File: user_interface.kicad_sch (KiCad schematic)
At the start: 11 parts, among them J4 B4B-XH-AM, J6 Conn_01x05, Q2 BC817, Q3 BC817

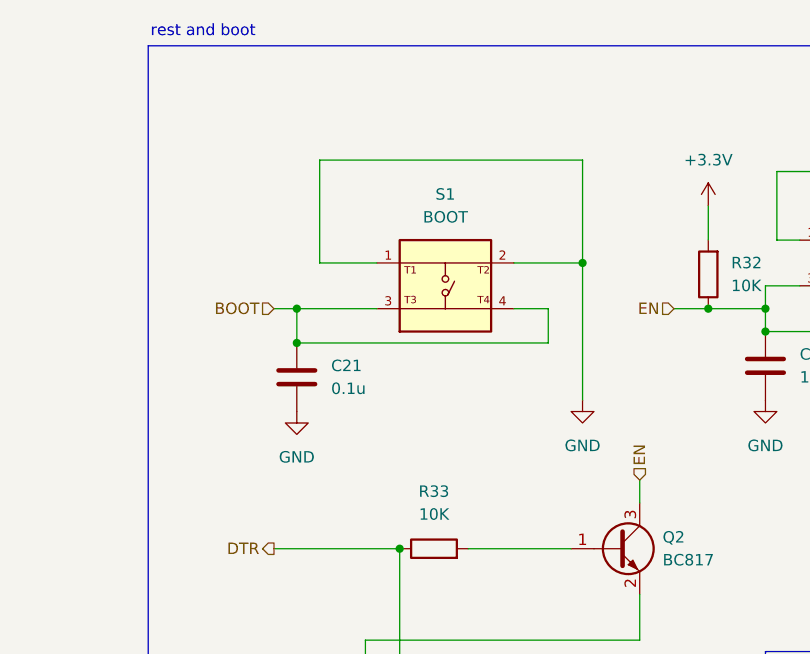
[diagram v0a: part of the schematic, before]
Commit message: intial_PCB
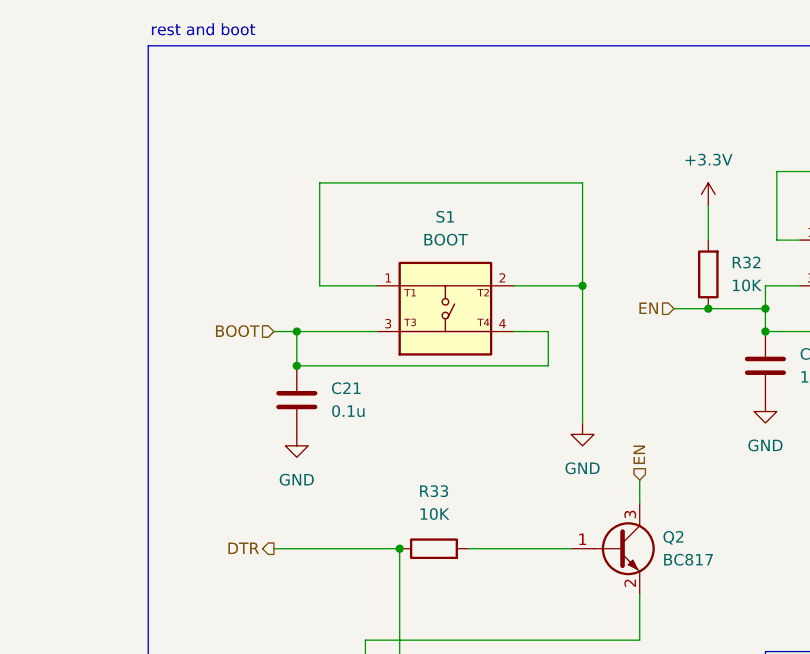
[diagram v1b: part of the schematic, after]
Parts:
- S1, S2: footprint USLPT2819DT2TR:SW_USLPT2819DT2TR -> Footprints:SW_USLPT2819DT2TR
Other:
- moved on the sheet: C21, S1
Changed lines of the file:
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@@
 	)
 	(junction
-		(at 163.83 58.42)
+		(at 163.83 60.96)
 		(diameter 0)
 		(color 0 0 0 0)
@@
 	)
 	(junction
-		(at 132.08 63.5)
+		(at 132.08 66.04)
 		(diameter 0)
 		(color 0 0 0 0)
@@
 	)
 	(junction
-		(at 132.08 67.31)
+		(at 132.08 69.85)
 		(diameter 0)
 		(color 0 0 0 0)
@@
 	(wire
 		(pts
-			(xy 163.83 58.42) (xy 163.83 73.66)
+			(xy 163.83 60.96) (xy 163.83 76.2)
 		)
 		(stroke
@@
 	(wire
 		(pts
-			(xy 129.54 63.5) (xy 132.08 63.5)
+			(xy 129.54 66.04) (xy 132.08 66.04)
 		)
 		(stroke
@@
 	(wire
 		(pts
-			(xy 134.62 46.99) (xy 163.83 46.99)
+			(xy 134.62 49.53) (xy 163.83 49.53)
 		)
 		(stroke
@@
 	(wire
 		(pts
-			(xy 140.97 58.42) (xy 134.62 58.42)
+			(xy 140.97 60.96) (xy 134.62 60.96)
 		)
 		(stroke
@@
 	(wire
 		(pts
-			(xy 132.08 63.5) (xy 140.97 63.5)
+			(xy 132.08 66.04) (xy 140.97 66.04)
 		)
 		(stroke
@@
 	(wire
 		(pts
-			(xy 163.83 46.99) (xy 163.83 58.42)
-		)
-		(stroke
-			(width 0)
-			(type default)
-		)
-	)
-	(wire
-		(pts
-			(xy 160.02 67.31) (xy 132.08 67.31)
-		)
-		(stroke
-			(width 0)
-			(type default)
-		)
-	)
-	(wire
-		(pts
-			(xy 132.08 63.5) (xy 132.08 67.31)
-		)
-		(stroke
-			(width 0)
-			(type default)
-		)
-	)
-	(wire
-		(pts
-			(xy 156.21 58.42) (xy 163.83 58.42)
+			(xy 163.83 49.53) (xy 163.83 60.96)
+		)
+		(stroke
+			(width 0)
+			(type default)
+		)
+	)
+	(wire
+		(pts
+			(xy 160.02 69.85) (xy 132.08 69.85)
+		)
+		(stroke
+			(width 0)
+			(type default)
+		)
+	)
+	(wire
+		(pts
+			(xy 132.08 66.04) (xy 132.08 69.85)
+		)
+		(stroke
+			(width 0)
+			(type default)
+		)
+	)
+	(wire
+		(pts
+			(xy 156.21 60.96) (xy 163.83 60.96)
 		)
 		(stroke
@@
 	(wire
 		(pts
-			(xy 134.62 58.42) (xy 134.62 46.99)
-		)
-		(stroke
-			(width 0)
-			(type default)
-		)
-	)
-	(wire
-		(pts
-			(xy 156.21 63.5) (xy 160.02 63.5)
-		)
-		(stroke
-			(width 0)
-			(type default)
-		)
-	)
-	(wire
-		(pts
-			(xy 160.02 63.5) (xy 160.02 67.31)
+			(xy 134.62 60.96) (xy 134.62 49.53)
+		)
+		(stroke
+			(width 0)
+			(type default)
+		)
+	)
+	(wire
+		(pts
+			(xy 156.21 66.04) (xy 160.02 66.04)
+		)
+		(stroke
+			(width 0)
+			(type default)
+		)
+	)
+	(wire
+		(pts
+			(xy 160.02 66.04) (xy 160.02 69.85)
 		)
 		(stroke
@@
 	(hierarchical_label "BOOT"
 		(shape input)
-		(at 129.54 63.5 180)
+		(at 129.54 66.04 180)
 		(effects
 			(font
@@
 	(symbol
 		(lib_id "USLPT2819DT2TR:USLPT2819DT2TR")
-		(at 148.59 60.96 0)
+		(at 148.59 63.5 0)
 		(unit 1)
 		(exclude_from_sim no)
@@
 		(fields_autoplaced yes)
 		(property "Reference" "S1"
-			(at 148.59 50.8 0)
+			(at 148.59 53.34 0)
 			(effects
 				(font
@@
 		)
 		(property "Value" "BOOT"
-			(at 148.59 53.34 0)
-			(effects
-				(font
-					(size 1.27 1.27)
-				)
-			)
-		)
-		(property "Footprint" "USLPT2819DT2TR:SW_USLPT2819DT2TR"
-			(at 148.59 60.96 0)
+			(at 148.59 55.88 0)
+			(effects
+				(font
+					(size 1.27 1.27)
+				)
+			)
+		)
+		(property "Footprint" "Footprints:SW_USLPT2819DT2TR"
+			(at 148.59 63.5 0)
 			(effects
 				(font
@@
 		)
 		(property "Datasheet" ""
-			(at 148.59 60.96 0)
+			(at 148.59 63.5 0)
 			(effects
 				(font
@@
 		)
 		(property "Description" ""
-			(at 148.59 60.96 0)
+			(at 148.59 63.5 0)
 			(effects
 				(font
@@
 		)
 		(property "MF" "TE Connectivity"
-			(at 148.59 60.96 0)
+			(at 148.59 63.5 0)
 			(effects
 				(font
@@
 		)
 		(property "Description_1" "Tactile Switch SPST-NO Top Actuated Surface Mount"
-			(at 148.59 60.96 0)
+			(at 148.59 63.5 0)
 			(effects
 				(font
@@
 		)
 		(property "Package" "None"
-			(at 148.59 60.96 0)
+			(at 148.59 63.5 0)
 			(effects
 				(font
@@
 		)
 		(property "Price" "None"
-			(at 148.59 60.96 0)
+			(at 148.59 63.5 0)
 			(effects
 				(font
@@
 		)
 		(property "Check_prices" "https://www.snapeda.com/parts/USLPT2819DT2TR/TE+Connectivity+ALCOSWITCH+Switches/view-part/?ref=eda"
-			(at 148.59 60.96 0)
+			(at 148.59 63.5 0)
 			(effects
 				(font
@@
 		)
 		(property "STANDARD" "Manufacturer Recommendations"
-			(at 148.59 60.96 0)
+			(at 148.59 63.5 0)
 			(effects
 				(font
@@
 		)
 		(property "PARTREV" "P"
-			(at 148.59 60.96 0)
+			(at 148.59 63.5 0)
 			(effects
 				(font
@@
 		)
 		(property "SnapEDA_Link" "https://www.snapeda.com/parts/USLPT2819DT2TR/TE+Connectivity+ALCOSWITCH+Switches/view-part/?ref=snap"
-			(at 148.59 60.96 0)
+			(at 148.59 63.5 0)
 			(effects
 				(font
@@
 		)
 		(property "MP" "USLPT2819DT2TR"
-			(at 148.59 60.96 0)
+			(at 148.59 63.5 0)
 			(effects
 				(font
@@
 		)
 		(property "Availability" "In Stock"
-			(at 148.59 60.96 0)
+			(at 148.59 63.5 0)
 			(effects
 				(font
@@
 		)
 		(property "MANUFACTURER" "TE CONNECTIVITY"
-			(at 148.59 60.96 0)
+			(at 148.59 63.5 0)
 			(effects
 				(font
@@
 	(symbol
 		(lib_id "power:GND")
-		(at 132.08 74.93 0)
+		(at 132.08 77.47 0)
 		(unit 1)
 		(exclude_from_sim no)
@@
 		(fields_autoplaced yes)
 		(property "Reference" "#PWR055"
-			(at 132.08 81.28 0)
+			(at 132.08 83.82 0)
 			(effects
 				(font
@@
 		)
 		(property "Value" "GND"
-			(at 132.08 80.01 0)
+			(at 132.08 82.55 0)
 			(effects
 				(font
@@
 		)
 		(property "Footprint" ""
-			(at 132.08 74.93 0)
+			(at 132.08 77.47 0)
 			(effects
 				(font
@@
 		)
 		(property "Datasheet" ""
-			(at 132.08 74.93 0)
+			(at 132.08 77.47 0)
 			(effects
 				(font
@@
 		)
 		(property "Description" "Power symbol creates a global label with name \"GND\" , ground"
-			(at 132.08 74.93 0)
+			(at 132.08 77.47 0)
 			(effects
 				(font
@@
 			)
 		)
-		(property "Footprint" "USLPT2819DT2TR:SW_USLPT2819DT2TR"
+		(property "Footprint" "Footprints:SW_USLPT2819DT2TR"
 			(at 195.58 58.42 0)
 			(effects
@@
 	(symbol
 		(lib_id "power:GND")
-		(at 163.83 73.66 0)
+		(at 163.83 76.2 0)
 		(unit 1)
 		(exclude_from_sim no)
@@
 		(fields_autoplaced yes)
 		(property "Reference" "#PWR050"
-			(at 163.83 80.01 0)
+			(at 163.83 82.55 0)
 			(effects
 				(font
@@
 		)
 		(property "Value" "GND"
-			(at 163.83 78.74 0)
+			(at 163.83 81.28 0)
 			(effects
 				(font
@@
 		)
 		(property "Footprint" ""
-			(at 163.83 73.66 0)
+			(at 163.83 76.2 0)
 			(effects
 				(font
@@
 		)
 		(property "Datasheet" ""
-			(at 163.83 73.66 0)
+			(at 163.83 76.2 0)
 			(effects
 				(font
@@
 		)
 		(property "Description" "Power symbol creates a global label with name \"GND\" , ground"
-			(at 163.83 73.66 0)
+			(at 163.83 76.2 0)
 			(effects
 				(font
@@
 	(symbol
 		(lib_id "Device:C")
-		(at 132.08 71.12 0)
+		(at 132.08 73.66 0)
 		(unit 1)
 		(exclude_from_sim no)
@@
 		(fields_autoplaced yes)
 		(property "Reference" "C21"
-			(at 135.89 69.8499 0)
+			(at 135.89 72.3899 0)
 			(effects
 				(font
@@
 		)
 		(property "Value" "0.1u"
-			(at 135.89 72.3899 0)
+			(at 135.89 74.9299 0)
 			(effects
 				(font
@@
 		)
 		(property "Footprint" "Capacitor_SMD:C_0805_2012Metric"
-			(at 133.0452 74.93 0)
+			(at 133.0452 77.47 0)
 			(effects
 				(font
@@
 		)
 		(property "Datasheet" "~"
-			(at 132.08 71.12 0)
+			(at 132.08 73.66 0)
 			(effects
 				(font
@@
 		)
 		(property "Description" "Unpolarized capacitor"
-			(at 132.08 71.12 0)
-			(effects
-				(font
+			(at 132.08 73.66 0)
+			(effects
+				(font
